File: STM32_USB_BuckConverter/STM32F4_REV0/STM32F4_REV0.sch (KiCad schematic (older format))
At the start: 50 parts, among them J1 Screw_Terminal_01x02, J2 SWD, J3 Conn_01x04, J4 Conn_01x04, J5 USB_B_Micro, Q1 AO3401A, SW1 SW_SPDT, U1 MP2359DJ-LF-Z, U2 STM32F405RGT6, U3 USBLC6-2SC6, Y1 16MHz

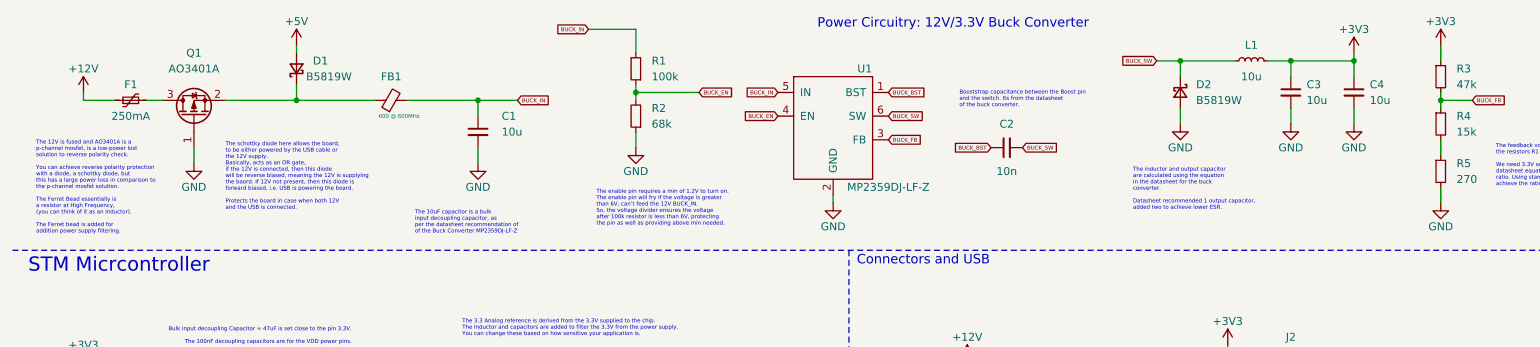
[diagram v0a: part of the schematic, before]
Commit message: Finished layout of MCU.
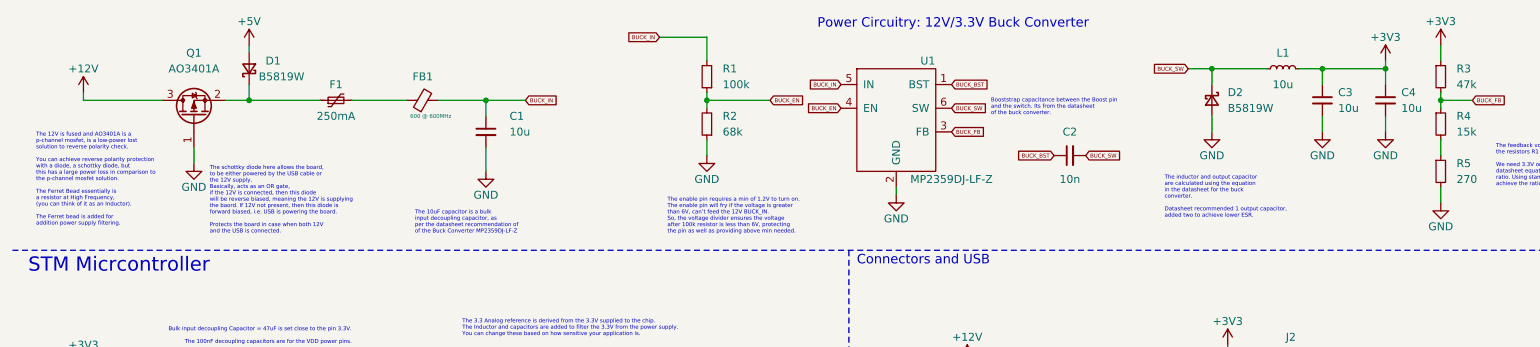
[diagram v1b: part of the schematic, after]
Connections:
- net +12V: now also Q1.3 (D); no longer F1.1
- net at F1.2: now also FB1.1; no longer Q1.3 (D)
- net at D1.1 (K), Q1.2 (S): now also F1.1; no longer FB1.1
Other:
- moved on the sheet: C1, C2, C3, C4, D1, D2, F1, FB1, L1, R1, R2, U1
